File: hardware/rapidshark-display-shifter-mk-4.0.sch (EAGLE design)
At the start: 11 parts, among them U1 ADAFRUIT_FEATHER_SHIELD

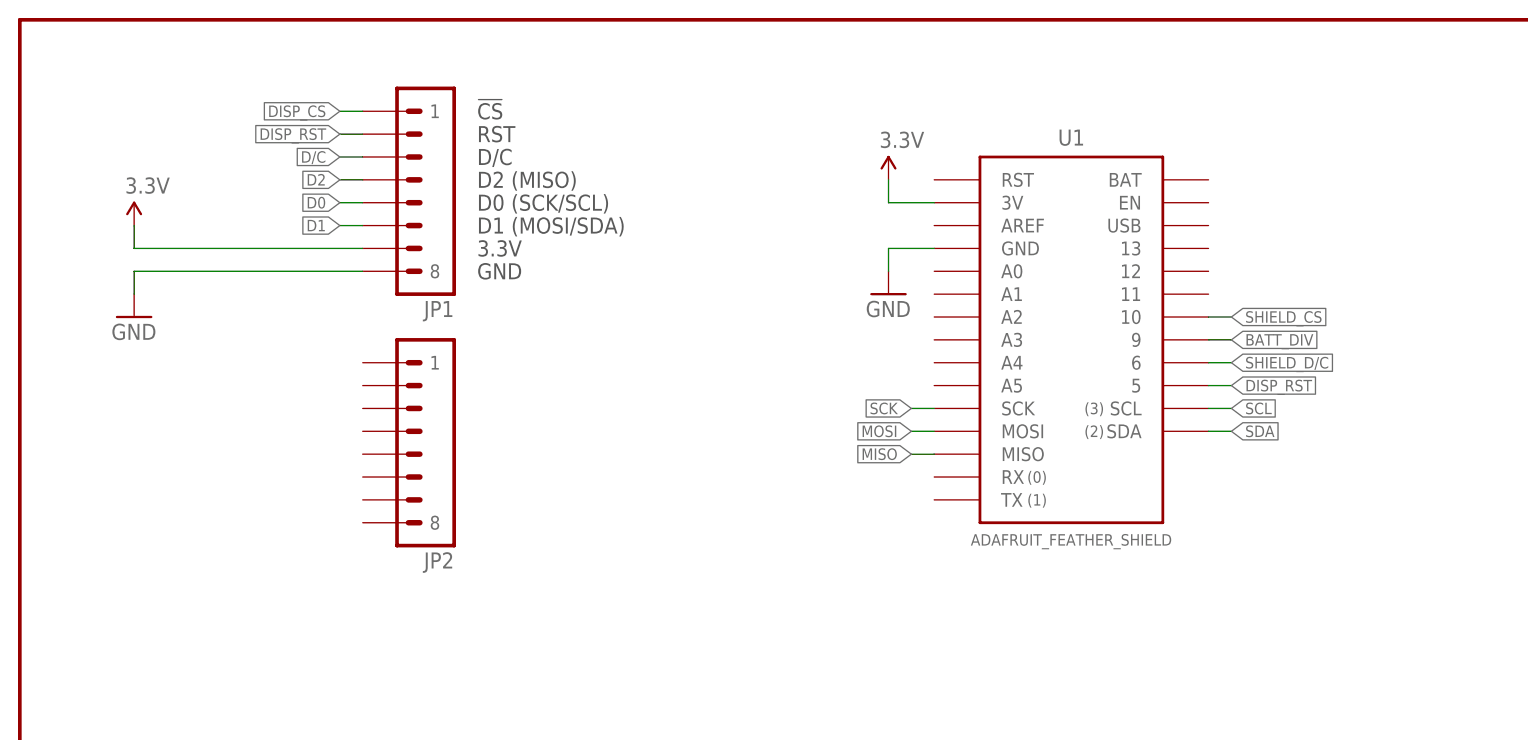
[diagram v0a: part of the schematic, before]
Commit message: adding these to commit to log before shifting to another repo
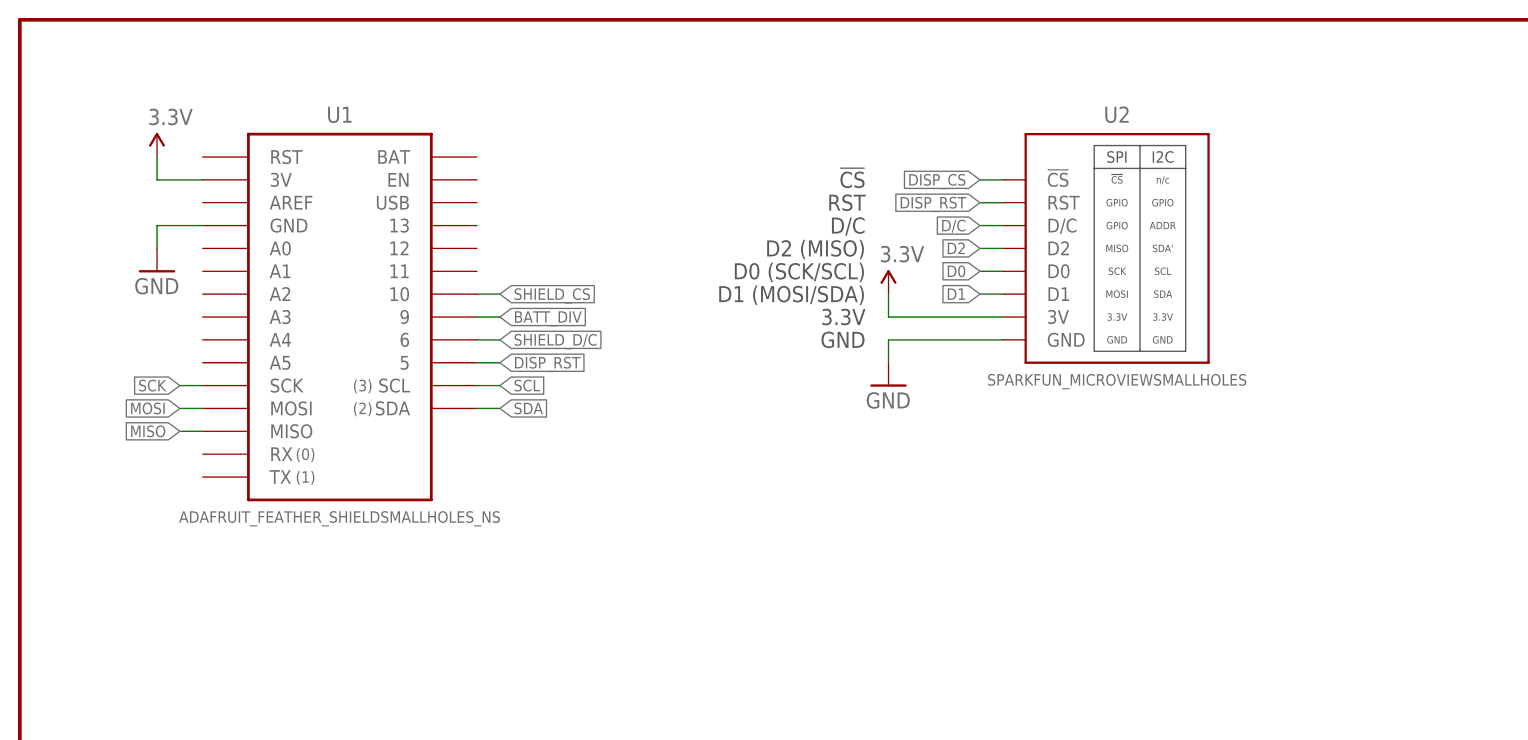
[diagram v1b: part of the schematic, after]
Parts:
- removed JP1, JP2: M081X08, A_butts:M081X08
- added U2: SPARKFUN_MICROVIEWSMALLHOLES, a_parts:SPARKFUN_MICROVIEWSMALLHOLES
- U1: value ADAFRUIT_FEATHER_SHIELD -> ADAFRUIT_FEATHER_SHIELDSMALLHOLES_NS; device a_parts:ADAFRUIT_FEATHER_SHIELD -> a_parts:ADAFRUIT_FEATHER_SHIELDSMALLHOLES_NS
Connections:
- net 3.3V: now also U2.3V; no longer JP1.7
- net D/C: now also U2.D/C; no longer JP1.3
- net D0: now also U2.D0; no longer JP1.5
- net D1: now also U2.D1; no longer JP1.6
- net D2: now also U2.D2; no longer JP1.4
- net DISP_CS: now also U2.!CS; no longer JP1.1
- net DISP_RST: now also U2.RST; no longer JP1.2
- net GND: now also U2.GND; no longer JP1.8
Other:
- moved on the sheet: U1
